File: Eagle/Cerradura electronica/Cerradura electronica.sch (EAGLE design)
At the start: 35 parts, among them IC1 LD117AS50TR, Q1 2N3904, Q2 IRF540NS, U1 ATMEGA328P_TQFP

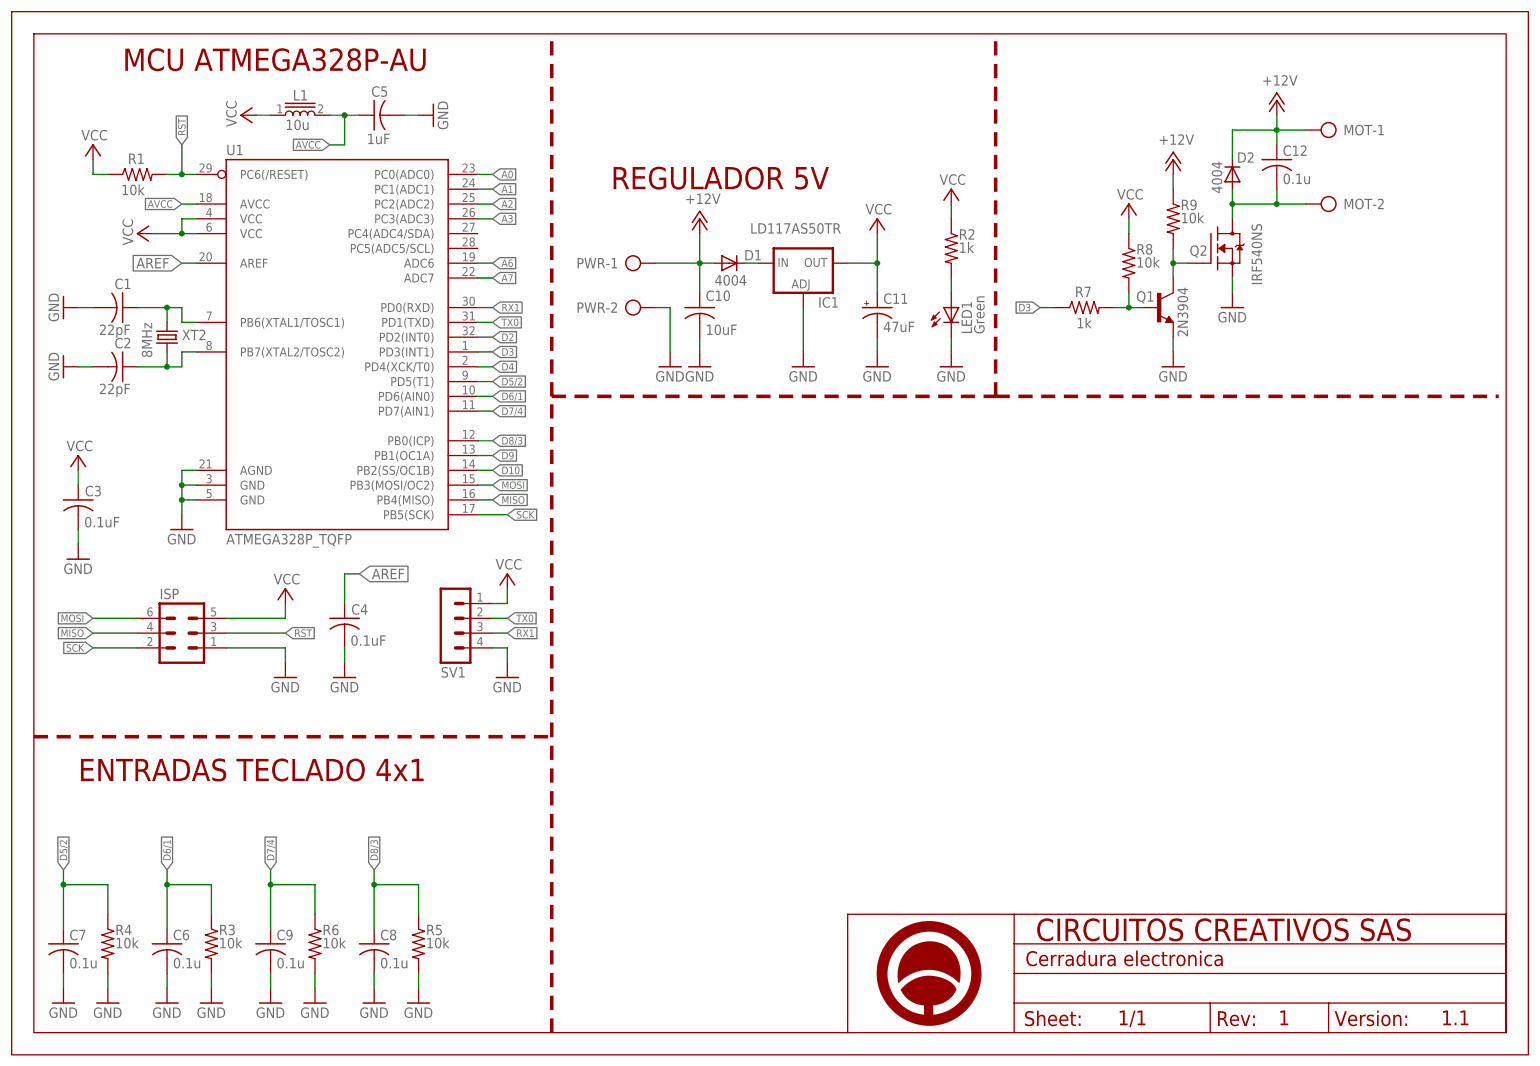
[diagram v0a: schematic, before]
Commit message: Terminado el SCH, inicio del BRD
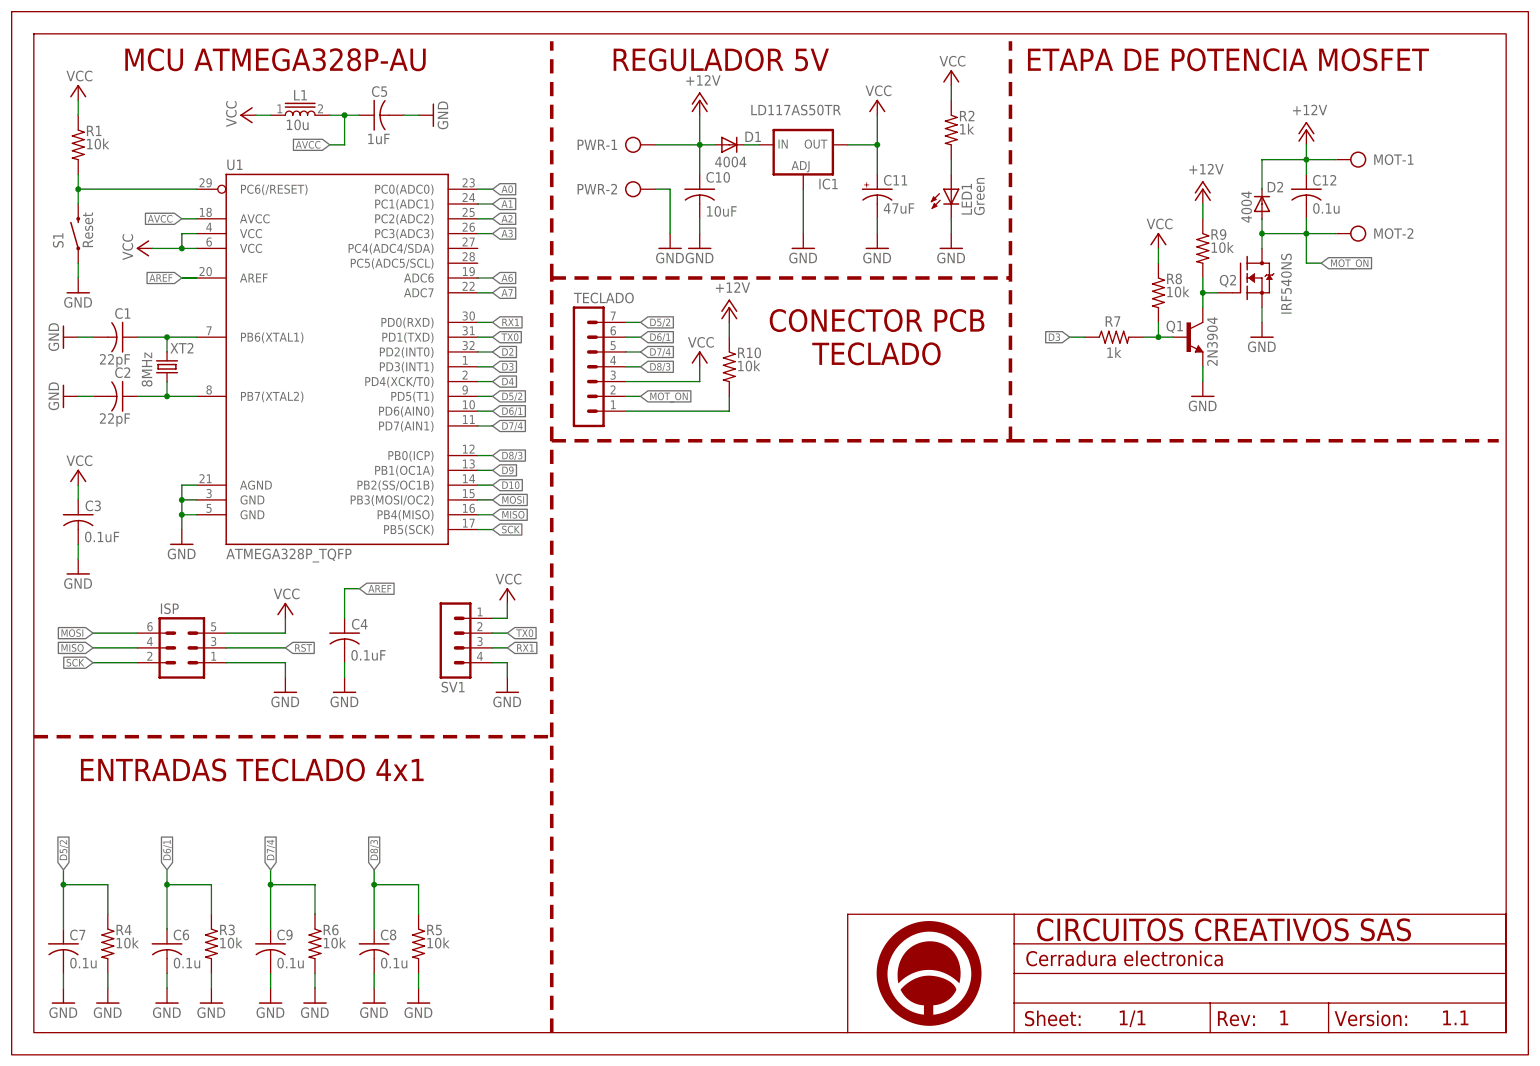
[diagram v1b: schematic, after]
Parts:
- added R10: 10k, rcl:R-US_R1206
- added S1: Reset, Testing:SWITCH-MOMENTARY-2-SMD-1101NE
- added TECLADO: (no value), con-lstb:MA07-1
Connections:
- removed net N$5: C12.2, D2.A, MOT-2.KL, Q2.D
- new net MOT_ON: C12.2, D2.A, MOT-2.KL, Q2.D, TECLADO.2
- new net N$11: R10.2, TECLADO.1
- new net RESET: R1.2, S1.2, U1.PC6(/RESET)
- net +12V: now also R10.1
- net D5/2: now also TECLADO.7
- net D6/1: now also TECLADO.6
- net D7/4: now also TECLADO.5
- net D8/3: now also TECLADO.4
- net GND: now also S1.1
- net OS1: now also U1.PB6(XTAL1); no longer U1.PB6(XTAL1/TOSC1)
- net OS2: now also U1.PB7(XTAL2); no longer U1.PB7(XTAL2/TOSC2)
- net RST: no longer R1.2, U1.PC6(/RESET)
- net VCC: now also TECLADO.3
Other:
- note added: "CONECTOR PCB TECLADO"
- note added: "ETAPA DE POTENCIA MOSFET"
- moved on the sheet: C1, C10, C11, C12, C2, C3, C4, D1, D2, IC1, ISP, LED1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
